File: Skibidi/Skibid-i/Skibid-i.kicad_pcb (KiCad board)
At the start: 2 copper layers, 140 x 104.8 mm, 62 parts, among them IC1 TEENSY_4.1, J1 Conn_01x02_Pin, J10 Screw_Terminal_01x04, J11 Screw_Terminal_01x04, J12 Screw_Terminal_01x03, J13 P78E05-1000, J14 Conn_01x02_Pin, J15 Conn_01x03_Pin, J16 Conn_01x02_Pin, J17 Conn_01x08_Pin, J18 Conn_01x02_Pin, J19 Conn_01x02_Pin, J2 Screw_Terminal_01x03, J21 Motor1, J22 Motor2, J3 Screw_Terminal_01x03, J4 Screw_Terminal_01x03, J5 Screw_Terminal_01x03, J6 Screw_Terminal_01x03, J7 Screw_Terminal_01x03, J8 Screw_Terminal_01x03, J9 Screw_Terminal_01x03, Q1 WL-OCPT_SERIES_357, Q2 WL-OCPT_SERIES_357, Q3 WL-OCPT_SERIES_357, Q4 WL-OCPT_SERIES_357, Q5 WL-OCPT_SERIES_357, Q6 WL-OCPT_SERIES_357, Q7 WL-OCPT_SERIES_357, SW2 210-4MS, U10 TXB0108PWR

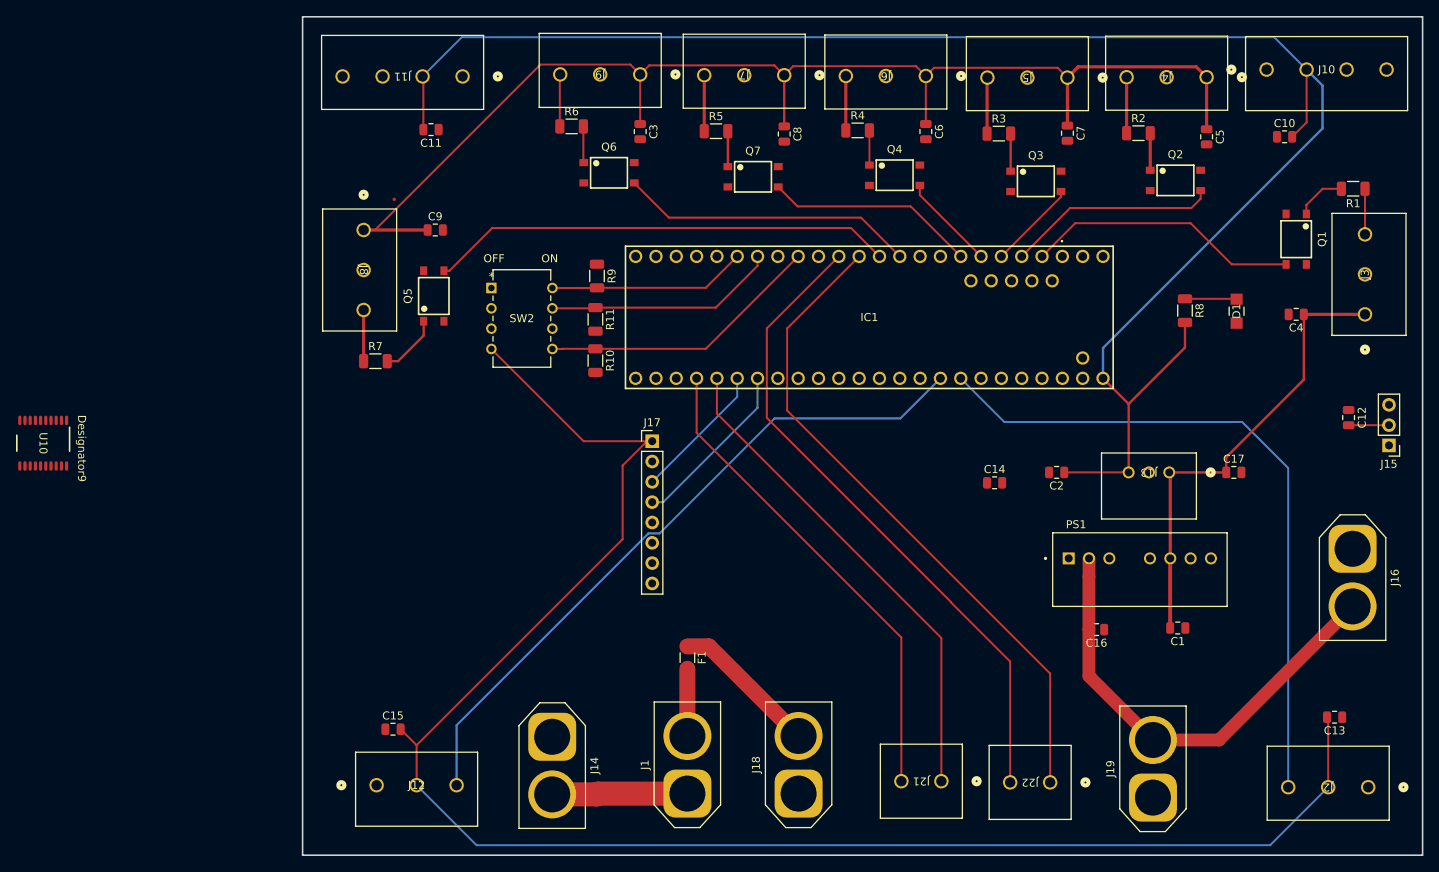
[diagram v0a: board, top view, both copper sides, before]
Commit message: layout
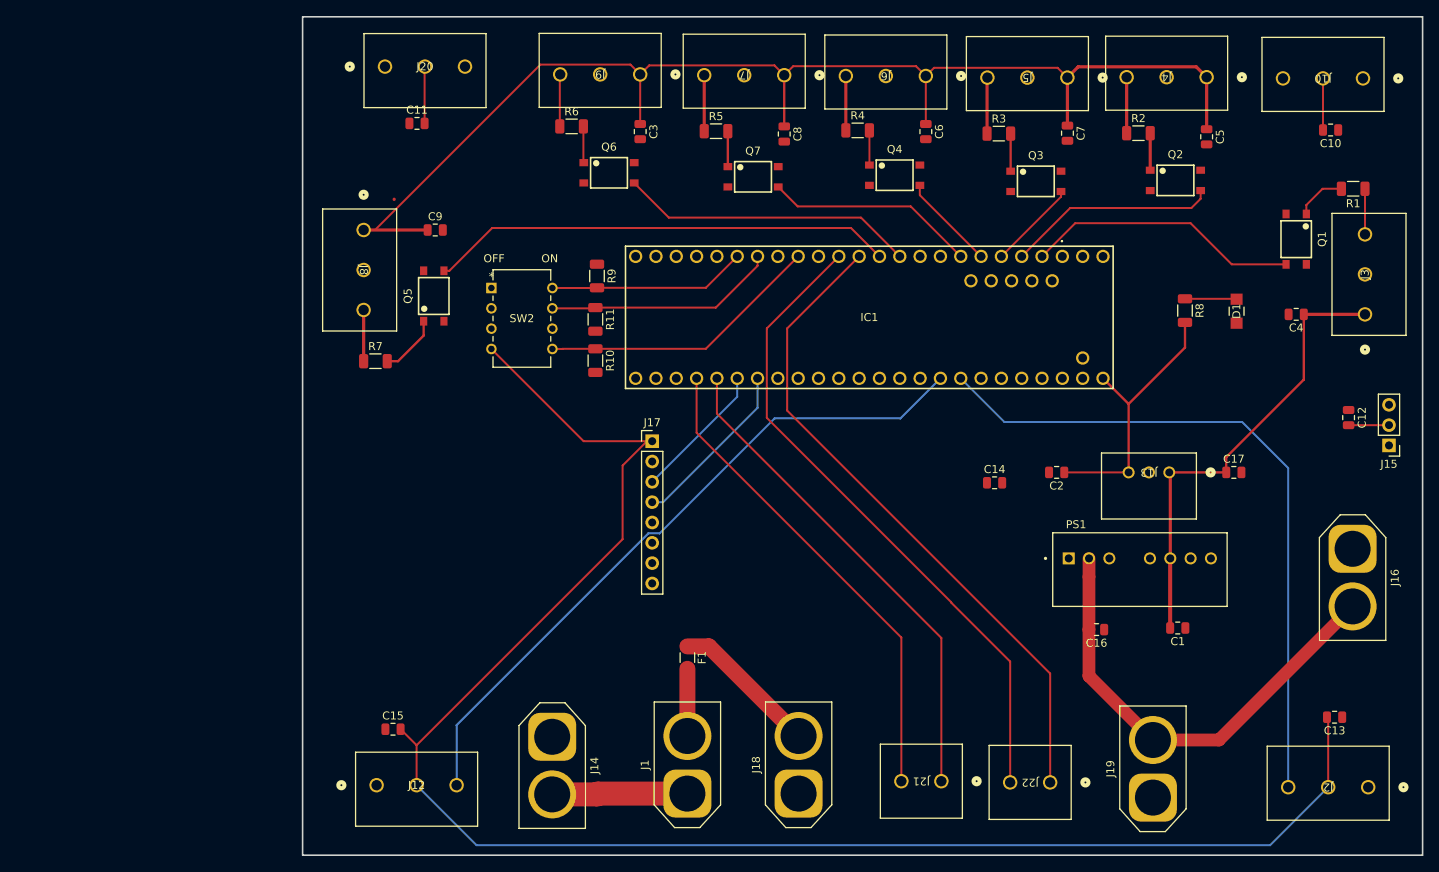
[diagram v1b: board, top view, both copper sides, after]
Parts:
- removed J11: Screw_Terminal_01x04, askibidi:Screwterimal4
- removed U10: TXB0108PWR, askibidi:levelshifter
- added J20: Screw_Terminal_01x03, askibidi:Screwterimanl3, F.Cu at (144.8, 35.7)
- J10: value Screw_Terminal_01x04 -> Screw_Terminal_01x03; footprint askibidi:Screwterimal4 -> askibidi:Screwterimanl3
- moved J10 12.1 mm to (267.1, 37.2), turned to 180 degrees
- moved C10 5.82 mm to (263.0, 43.6), turned to 180 degrees
- moved C11 1.91 mm to (148.8, 42.8), turned to 0 degrees
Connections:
- C10 pad 2: +5V -> +3.3V
- C11 pad 2: +5V -> +3.3V
- IC1 pad 14: LN1A -> LN1
- IC1 pad 15: LN2A -> LN2
- IC1 pad 16: LN3A -> LN3
- IC1 pad 17: LN4A -> LN4
- IC1 pad 18: LN5 -> unconnected-(IC1-A4-Pad18)
- IC1 pad 19: LN6 -> unconnected-(IC1-A5-Pad19)
- J10 pad 2: +5V -> +3.3V
- J12 pad 3: LN5 -> LN3
- J2 pad 3: LN6 -> LN4
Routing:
- net +5V: track 215.1 -> 34.3 mm
- net LN5: track 85.9 -> 0.00 mm
- net LN3: track 0.00 -> 85.9 mm
- net LN6: track 85.5 -> 0.00 mm
- net LN4: track 0.00 -> 85.5 mm
- net +3.3V: track 217.2 -> 230.8 mm
